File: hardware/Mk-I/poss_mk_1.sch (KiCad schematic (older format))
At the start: 34 parts, among them SW1 SW_PUSH, SW10 SW_PUSH, SW11 SW_PUSH, SW12 SW_PUSH, SW13 SW_PUSH, SW14 SW_PUSH, SW15 SW_PUSH, SW16 SW_PUSH, SW18 SW_PUSH, SW19 SW_PUSH, SW2 SW_PUSH, SW20 SW_PUSH, SW21 SW_PUSH, SW22 SW_PUSH, SW3 SW_PUSH, SW4 SW_PUSH, SW5 SW_PUSH, SW6 SW_PUSH, SW7 SW_PUSH, SW8 SW_PUSH, SW9 SW_PUSH, U6 encoder_and_switch, U7 encoder_and_switch

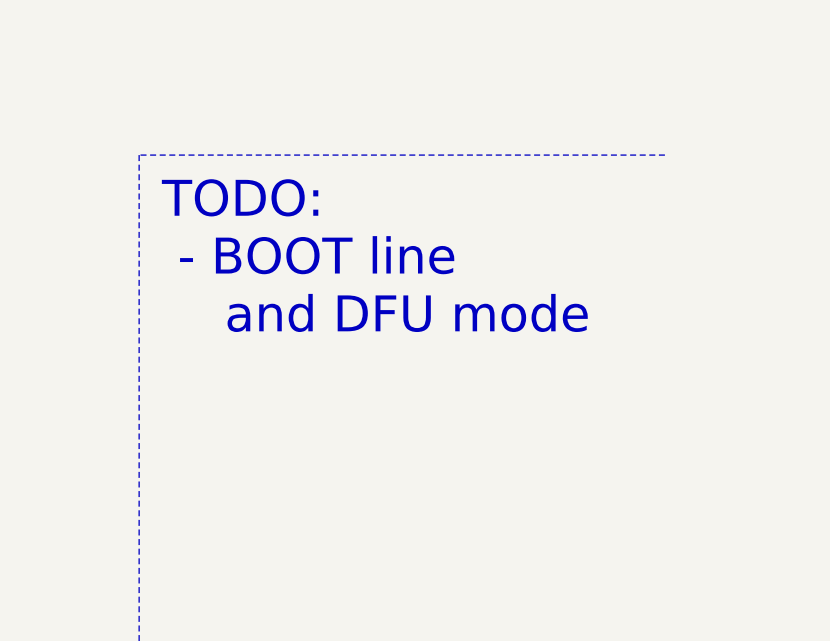
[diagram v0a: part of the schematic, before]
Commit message: Update TODO list
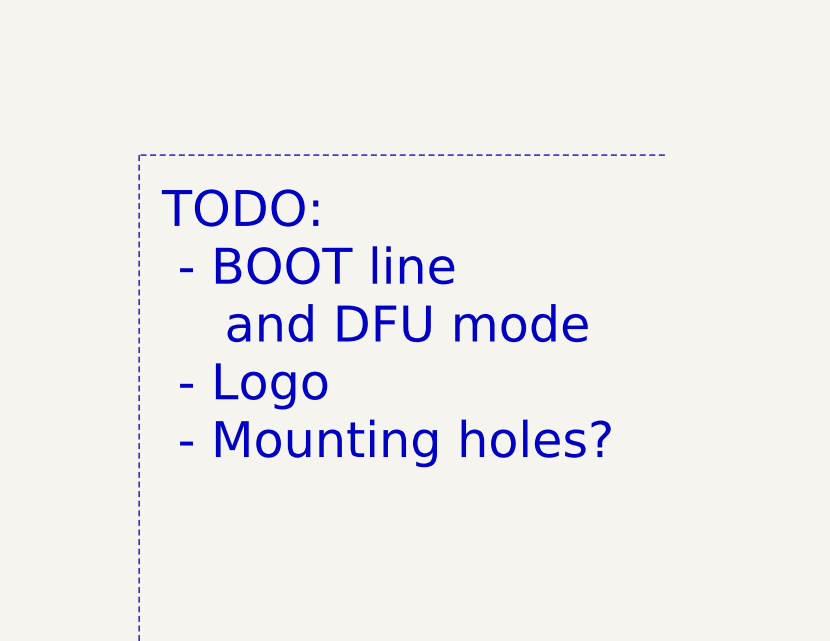
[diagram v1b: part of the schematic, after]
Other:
- note added: "TODO:\n - BOOT line \n and DFU mode\n - Logo\n - Mounting holes?"
- note removed: "TODO:\n - BOOT line \n and DFU mode"
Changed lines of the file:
@@
 F1 "audio.sch" 60
 $EndSheet
-Text Notes 8950 4900 0    157  ~ 0
-TODO:\n - BOOT line \n    and DFU mode
+Text Notes 8950 5450 0    157  ~ 0
+TODO:\n - BOOT line \n    and DFU mode\n - Logo\n - Mounting holes?
 Text GLabel 4850 5700 0    60   Input ~ 0
 WAKEUP
